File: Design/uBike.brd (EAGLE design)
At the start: 55 x 85 mm, 86 parts, among them J10 455-1750-1-ND, J5 C167321, J6 C111196, J9 CONN_08, Q1 B772, Q2 B772, U1 RA-02_LORA, U10 MAX17048, U2 RP2040, U3 W25Q128JVSIQ, U5 PAM2401, U6 AMS1117-3.3, U8 MCP73831, Y1 12MHz

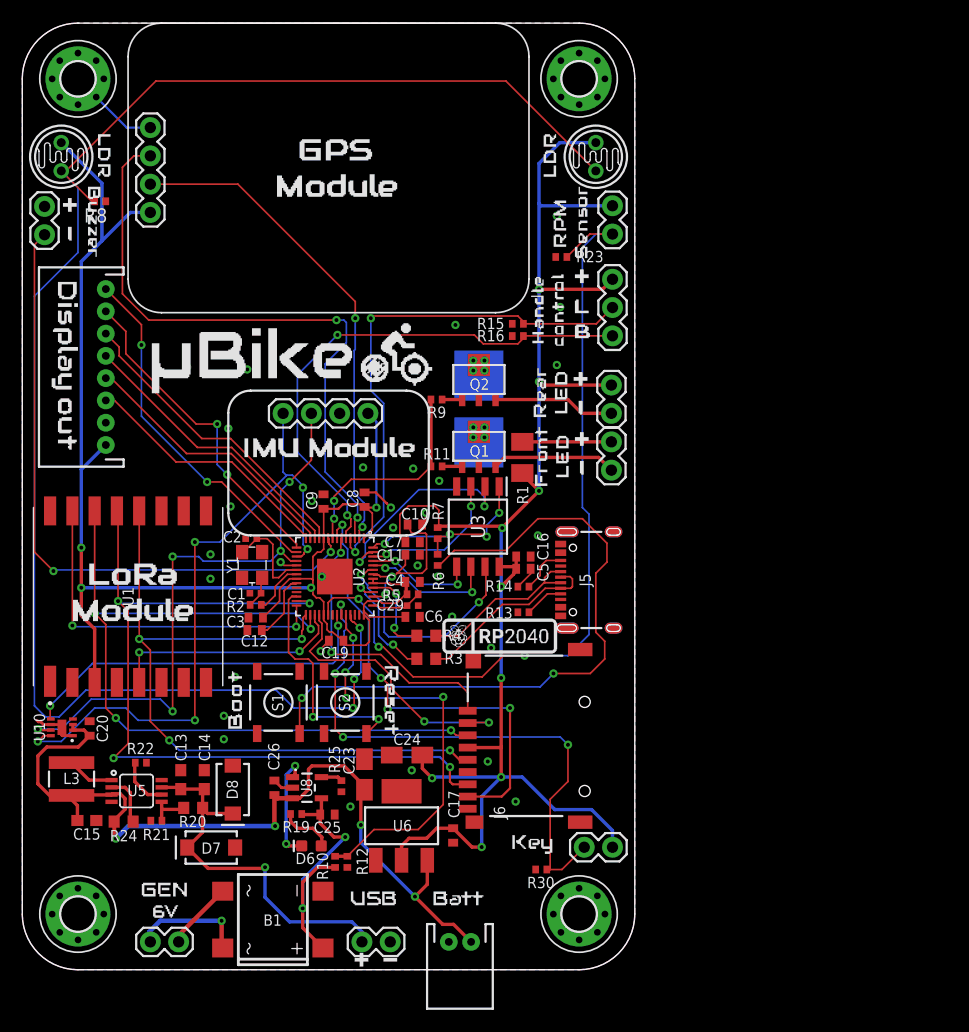
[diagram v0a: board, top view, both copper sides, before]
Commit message: Frozen design for August 23 manufacturing batch
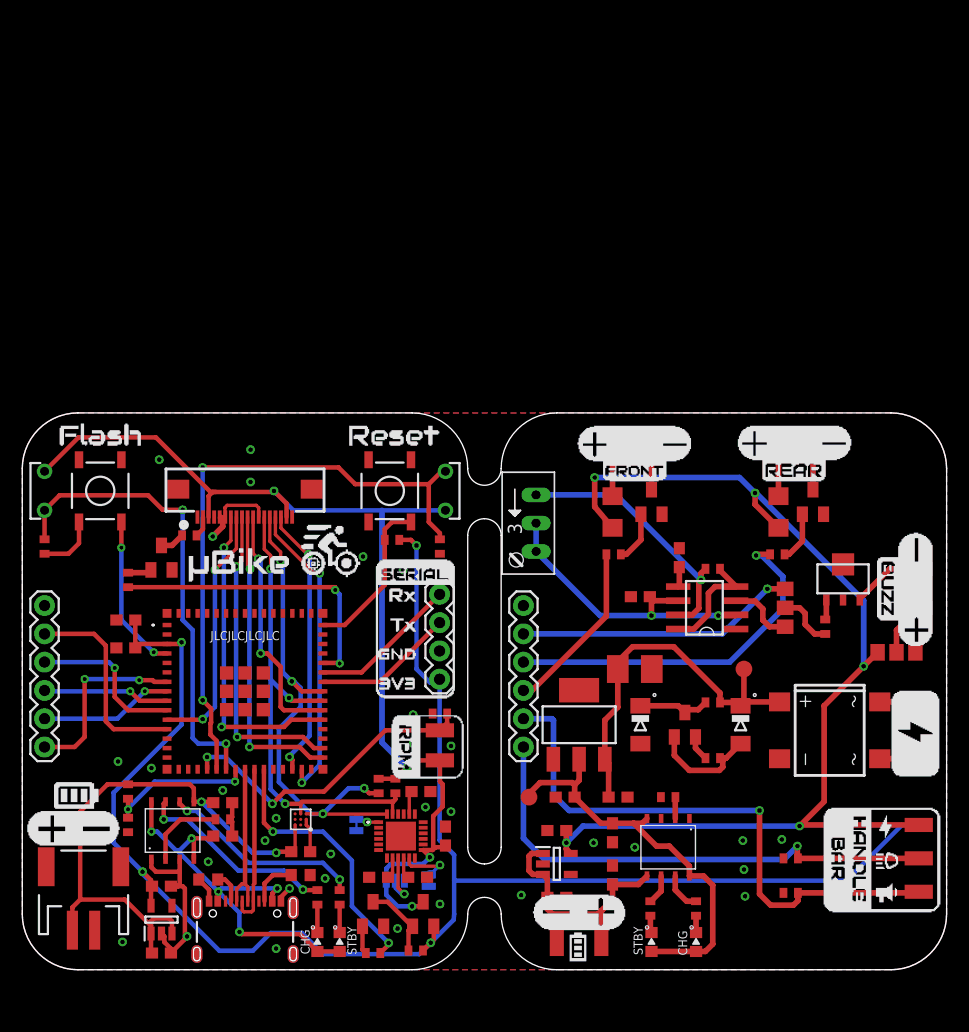
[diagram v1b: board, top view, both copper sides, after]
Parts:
- removed C20: 100nF, rcl:C0402
- removed C23, C24: 10uF, rcl:A/3216-18R
- removed C25, C26: 4.7uF, rcl:C0402
- removed C29: 2.2uF, SparkFun-Capacitors:0402-TIGHT
- removed D6: Yellow, SparkFun-LED:LED-0603
- removed D7, D8: B340A, SparkFun-DiscreteSemi:SMA-DIODE
- removed H1, H2, H3, H4: MOUNT-PAD-ROUND, SpaceDIY_connectors:3,0-PAD
- removed J10: 455-1750-1-ND, SparkFun-Connectors:1X03
- removed J11, J12, J13, J2, J3, J8: (no value), SparkFun-Connectors:1X02
- removed J14: (no value), SparkFun-Connectors:1X04
- removed J6: C111196, SparkFun-Connectors:MICROSD-EXTERNALPIN
- removed J9: CONN_08, SpaceDIY_connectors:JST-8-PTH
- removed L3: 2.2UH3A, SparkFun-Coils:INDUCTOR_4X4MM
- removed Q1, Q2: B772, User-Submitted:SOT89
- removed R30: 10k, rcl:R0402
- removed U$30: (no value), RP2040:RP2040_20
- removed U10: MAX17048, SparkFun-IC-Power:DFN-8
- removed U2: RP2040, RP2040:QFN-56
- removed U3: W25Q128JVSIQ, SamacSys_Parts:SOIC127P790X216-8N
- removed U5: PAM2401, SparkFun-IC-Power:MSOP8
- removed U6: AMS1117-3.3, SparkFun-IC-Power:SOT223
- removed U8: MCP73831, SparkFun-IC-Power:SOT23-5
- removed Y1: 12MHz, crystal-geyer_V1_0:3.2X2.5_KX-7
- added C18: 10uF, rcl:C0603
- added C40: 1uF, rcl:C0603
- added D1, D2: ZMM5V6-M, JLC PCB Basic Parts_loc:MELF-MLL34
- added IC1, IC4: TP4056, TP4056:SOT23-8
- added IC2, IC7: RT9080-33GJ5, SamacSys_Parts:SOT94P280X100-5N
- added IC3: MPU-6050, SpaceDIY_IC:MPU6050
- added IC5: LC709203F/MH, adafruit_sensor:WLCSP9
- added IC6: ESP32-S3-MINI-1U-N8, SpaceDIY_modules:ESP32S3MINI1UN8
- added IC8: TLC555CDR, adafruit:SO08
- added J18: (no value), SparkFun-Connectors:1X04
- added JMP1, JMP2: 0R-JUMPA, jump-0r-smd:A0R-JMP
- added LED1, LED3: Red, SpaceDIY_semiconductors:LED_0603
- added LED2, LED4: Green, SpaceDIY_semiconductors:LED_0603
- added PAD1, PAD10, PAD11, PAD12, PAD13, PAD14, PAD15, PAD2, PAD3, PAD4, PAD5, PAD6, PAD7, PAD8, PAD9: (no value), wirepad:SMD1,27-2,54
- added Q5: B772, User-Submitted:SOT89
- added R17, R28: 1k, SpaceDIY_passive_components:0402
- added R18: 10K, SpaceDIY_passive_components:0402
- added R26: 1.2k, SpaceDIY_passive_components:0402
- added R27: 1K, SpaceDIY_passive_components:0402
- added R29: 1M, SpaceDIY_passive_components:0402
- added R36, R37: 5.1k, rcl:R0603
- added SJ1: (no value), SparkFun:SJ_3_PASTE2&3
- added SJ2, SJ3: (no value), SparkFun:SJ_2S-TRACE
- added T1, T6: MMBT2222A, JLC PCB Basic Parts_loc:SOT23
- added T2: T_P-MOSFET_SI2301CDS-T1-GE3_VISHAY_SOT23-GSD, JLC PCB Basic Parts_loc:SOT23
- added T3, T4, T5: T_N-MOSFET_2N7002_CHANGJ_SOT23-GSD, JLC PCB Basic Parts_loc:SOT23
- added TP1, TP3: TPTP15R, testpad:TP15R
- added U$1: P169H002-CTP, SpaceDIY_connectors:FPC_18_0.5MM_BOTTOM
- C1: value 15pF -> 10uF; device SparkFun-Capacitors:0402-TIGHT -> rcl:C0603
- C10, C17, C4, C7, C8: value 100nF -> 10uF; device rcl:C0402 -> rcl:C0603
- C11: value 0.1uF -> 100nF; device rcl:C0402 -> rcl:C0603
- C12: value 2.2uF -> 2.2nF; device rcl:C0402 -> rcl:C0603
- C13, C15: value 22uF -> 0.1uF
- C14: value 22uF -> 10nF
- C16, C19: value 2.2uF -> 10uF; device rcl:C0402 -> rcl:C0603
- C2: value 15pF -> 100u; device SparkFun-Capacitors:0402-TIGHT -> SpaceDIY_passive_components:B/3528-21R
- C3: value 100nF -> 10u; device rcl:C0402 -> rcl:C0603
- C5: value 100nF -> 100n; device rcl:C0402 -> rcl:C0603
- C6: value 100nF -> 0.1uF; device rcl:C0402 -> rcl:C0603
- C9: value 100nF -> 10nF; device rcl:C0402 -> rcl:C0603
- J1: device SparkFun-Connectors:1X04 -> SpaceDIY_connectors:JST-2-SMD
- J4: device SparkFun-Connectors:1X02 -> SpaceDIY_connectors:1X06
- J5: value C167321 -> (none); device SparkFun-Connectors:USB-C-16P-4LAYER-ISOLATED -> SpaceDIY_connectors:1X06
- J7: value (none) -> USB-C; device SparkFun-Connectors:JST-2-PTH -> SparkFun-Connectors:USB-C-16P-4LAYER-ISOLATED
- PH1, PH2: value VT20N1 -> M9960_11A; device photo-elements:TO46-VT200 -> photo-elements:M9960
- R1: device rcl:M1206 -> rcl:R1206
- R10, R11, R15, R16, R23, R8, R9: device rcl:R0402 -> SpaceDIY_passive_components:0402
- R12: value 1k -> 1; device rcl:R0402 -> rcl:R1206
- R13: value 5.1k -> 10K; device rcl:R0402 -> SpaceDIY_passive_components:0402
- R14: value 5.1k -> 100; device rcl:R0402 -> SpaceDIY_passive_components:0402
- R19: value 1k -> (none); device rcl:R0402 -> pot:RJ9W
- R2: value 1k -> 10k; device rcl:R0402 -> SpaceDIY_passive_components:0402
- R20: value 750K -> 10K; device rcl:R0603 -> SpaceDIY_passive_components:0402
- R21: value 100k -> 10R; device rcl:R0402 -> SpaceDIY_passive_components:0402
- R22: value 100k -> 1k; device rcl:R0402 -> SpaceDIY_passive_components:0402
- R24: value 750K -> 10k; device rcl:R0603 -> SpaceDIY_passive_components:0402
- R25: value 2k -> 1M; device rcl:R0402 -> SpaceDIY_passive_components:0402
- R3: value 27 -> 1k; device rcl:R0603 -> SpaceDIY_passive_components:0402
- R4: value 27 -> 100; device rcl:R0603 -> SpaceDIY_passive_components:0402
- R5: value 200 -> 10k; device rcl:R0402 -> SpaceDIY_passive_components:0402
- R6: value 1k -> 1.2k; device rcl:R0402 -> SpaceDIY_passive_components:0402
- R7: value 10k -> 1K; device rcl:R0402 -> SpaceDIY_passive_components:0402
- S1: value MOMENTARY-SWITCH-SPST-SMD-5.2MM-TALL -> Flash; device SparkFun-Switches:TACTILE_SWITCH_SMD_5.2MM -> SpaceDIY_electromechanical:TACTILE_SWITCH_SMD_5.2MM
- S2: value MOMENTARY-SWITCH-SPST-SMD-5.2MM-TALL -> Reset; device SparkFun-Switches:TACTILE_SWITCH_SMD_5.2MM -> SpaceDIY_electromechanical:TACTILE_SWITCH_SMD_5.2MM
- U1: value RA-02_LORA -> AMS1117-5VSMD; device SpaceDIY_modules:MODULE_RA-02_LORA -> SpaceDIY_IC:SOT223
- moved J1 60.8 mm to (5.50, 7.50), turned to 180 degrees
- moved PH1 57.9 mm to (2.00, 43.0)
- moved R16 55.7 mm to (69.0, 6.90)
- moved R15 53.9 mm to (69.0, 10.0)
- moved B1 52.8 mm to (72.5, 21.5), turned to 270 degrees
- moved R12 49.9 mm to (67.9, 41.1), turned to 90 degrees
- moved PH2 45.7 mm to (38.0, 43.0), turned to 90 degrees
- moved R23 42.4 mm to (37.5, 23.0)
- moved U1 42.1 mm to (50.0, 22.0), turned to 0 degrees
- moved R7 40.9 mm to (60.5, 5.50)
- moved C1 40.8 mm to (53.0, 8.50), turned to 90 degrees
- moved C8 39.7 mm to (48.0, 6.50), turned to 0 degrees
- moved R24 37.6 mm to (37.5, 38.0), turned to 90 degrees
- moved C2 36.4 mm to (55.0, 27.0), turned to 180 degrees
- moved C3 36.3 mm to (53.5, 15.5), turned to 0 degrees
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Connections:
- removed net !RESET!: S2.3, U2.26
- removed net 1.1V: C10.1, C11.1, C12.1, U2.23, U2.45, U2.50
- removed net ADC0: R10.1, R12.1, U2.38
- removed net ADC1: PH1.2, PH2.2, R8.2, U2.39
- removed net ADC2: U2.40
- removed net ADC3: U2.41
- removed net AVDD: C29.1, R5.1, U2.43
- removed net BATT_ALERT: U10.5, U2.36
- removed net BOOT: R6.2, S1.3
- removed net DAT1: J6.8, U2.7
- removed net DAT2: J6.1, U2.6
- removed net EN_5: R24.1, U5.2
- removed net GPIO2: J10.2, R15.2, U2.4
- removed net GPIO20: U1.5, U2.31
- removed net GPIO21: J6.2, U2.32
- removed net GPIO22: J11.2, R23.2, U2.34
- removed net GPIO23: U2.35
- removed net GPIO25: J13.2, R30.2, U2.37
- removed net GPIO3: J10.3, R16.2, U2.5
- removed net GPIO6: R11.2, R9.2, U2.8
- removed net GPIO7: J12.1, U2.9
- removed net LCD_BL: J9.8, U2.16
- removed net LCD_RST: J9.7, U2.15
- removed net N$24: R20.1, R21.2, U5.5
- removed net N$25: L3.P$2, U5.1
- removed net N$26: R22.2, U5.6
- removed net QSPI-0: U2.53, U3.5
- removed net QSPI-1: U2.55, U3.2
- removed net QSPI-2: U2.54, U3.3
- removed net QSPI-3: U2.51, U3.7
- removed net QSPI-CLK: U2.52, U3.6
- removed net QSPI-CS: R6.1, R7.1, U2.56, U3.1
- removed net RX_GPS: J1.2, U2.2
- removed net SPI_0_CS: U1.15, U2.28
- removed net SPI_0_MISO: J6.7, U1.13, U2.27
- removed net SPI_0_MOSI: J6.3, U1.14, U2.30
- removed net SPI_0_SCK: J6.5, U1.12, U2.29
- removed net SPI_1_CS: J9.5, U2.12
- removed net SPI_1_MISO: J9.6, U2.11
- removed net SPI_1_MOSI: J9.3, U2.14
- removed net SPI_1_SCK: J9.4, U2.13
- removed net SWDCK: U2.24
- removed net SWDIO: U2.25
- removed net TX_GPS: J1.3, U2.3
- removed net USB_F_N1: R3.2, U2.46
- removed net USB_F_P1: R4.2, U2.47
- removed net USB_N: J5.A7, J5.B7, R3.1
- removed net USB_P: J5.A6, J5.B6, R4.1
- removed net V_BATT: C15.1, C20.1, C23.+, C26.1, J7.1, L3.P$1, R24.2, U10.2, U10.3, U5.3, U6.3, U8.3
- removed net V_IN: B1.+, C25.1, R10.2, R19.2, U8.4
- new net BAT_VOLT: IC6.22, R25.1, R29.2
- new net BUZZER: JMP2.2, R14.2
- new net BUZZ_PB: IC6.8, J4.2, J5.2, PAD15.1, R16.2
- new net CC3: J7.B5, R36.2
- new net CC4: J7.A5, R37.2
- new net D+: IC6.24, J7.A6, J7.B6
- new net D-: IC6.23, J7.A7, J7.B7
- new net IO0: IC6.4, S1.3
- new net LDR_LH: IC6.21, PH1.2, R8.2
- new net LDR_RH: IC6.20, PH2.2, R24.2
- new net LEDK: R21.1, U$1.2
- new net LED_FRONT: IC6.9, J4.3, J5.3, R11.2
- new net LED_PB: IC6.7, J4.1, J5.1, PAD14.1, R15.2
- new net LED_REAR: IC6.10, J4.4, J5.4, R9.2
- new net N$15: IC1.7, R7.2
- new net N$17: PAD12.1, Q5.3
- new net N$18: R3.2, T1.1
- new net N$19: JMP1.2, PAD11.1
- new net N$20: PAD1.1, R12.2
- new net N$33: R21.2, T6.3
- new net N$34: IC8.7, R17.2, R19.E
- new net N$35: C11.1, IC8.2, IC8.6, R19.A, R19.S
- new net N$36: IC8.3, JMP2.1
- new net N$37: C9.1, IC8.5
- new net N$38: IC3.11, SJ3.2
- new net N$39: IC3.1, SJ2.2
- new net N$40: C13.1, IC3.10
- new net N$41: C12.1, IC3.20
- new net N$43: C14.1, IC3.8
- new net N$44: IC3.9, SJ1.2
- new net N$46: R22.2, T6.1
- new net N$47: IC4.6, R28.2
- new net N$48: LED3.C, R27.1
- new net N$49: LED4.C, R28.1
- new net N$50: IC4.2, R26.2
- new net N$51: IC4.7, R27.2
- new net RPM: IC6.19, PAD10.1, R23.2
- new net RST: IC6.45, R13.1, S2.3
- new net RX: IC6.6
- new net RXD0: IC6.40, J18.4
- new net SENS: IC6.25, R3.1
- new net TFT_BL: IC6.41, R22.1
- new net TFT_CS: IC6.11, U$1.8
- new net TFT_DC: IC6.35, U$1.7
- new net TFT_MISO: IC6.33
- new net TFT_MOSI: IC6.31, U$1.10
- new net TFT_RST: IC6.36, U$1.11
- new net TFT_SCK: IC6.32, U$1.9
- new net TP_INT: IC6.28, U$1.16
- new net TP_RST: IC6.29, U$1.15
- new net TX: IC6.5
- new net TXD0: IC6.39, J18.3
- new net UC_BUZZER: IC6.12, J4.5, J5.5, JMP2.3
- new net VBAT: C16.1, C18.1, C40.1, IC4.5, IC5.A3, IC7.1, IC7.3, J1.1, R25.2
- new net VBAT_1: C1.1, C8.1, IC1.5, IC2.1, IC2.3, PAD5.1
- new net VBUS: C17.1, IC4.4, IC4.8, J7.VBUS1, J7.VBUS2, LED3.A, LED4.A
- new net VSENS: C15.1, IC3.13, PAD9.1, PH1.1, PH2.1, R18.1, R20.1, SJ1.1, T2.3, U$1.17, U$1.3
- new net V_BUZZ: IC8.4, IC8.8, R17.1
- new net V_DYN_UR: B1.+, C2.+, C3.1, D2.C, R4.1, TP1.TP, U1.3
- new net V_REG: C4.1, C5.1, IC1.4, IC1.8, LED1.A, LED2.A, TP3.TP, U1.2
- net 3.3V: now also C10.1, IC2.5, IC6.3, IC7.5, J18.1, JMP1.3, PAD13.1, R12.1, R13.2, R2.1, T2.2; no longer C16.1, C17.1, C24.+, C3.1, C4.1, C5.1, C8.1, C9.1, J1.1, J10.1, J11.1, J13.1, J14.1, J3.1, J6.4, J9.1, PH1.1, PH2.1, R5.2, R7.2, U1.3, U2.1, U2.10, U2.22, U2.33, U2.42, U2.44, U2.48, U2.49, U3.8, U6.2
- net 5V: now also JMP1.1; no longer C13.1, C14.1, D7.C, D8.C, J4.1, R20.2, U5.7
- net GND: now also C1.2, C18.2, C2.-, C40.2, D1.A, IC1.1, IC1.3, IC2.2, IC3.18, IC4.1, IC4.3, IC5.A1, IC5.B1, IC6.1, IC6.2, IC6.42, IC6.43, IC6.46, IC6.47, IC6.48, IC6.49, IC6.50, IC6.51, IC6.52, IC6.53, IC6.54, IC6.55, IC6.56, IC6.57, IC6.58, IC6.59, IC6.60, IC6.61, IC6.62, IC6.63, IC6.64, IC6.65, IC6.66, IC6.67, IC6.68, IC6.69, IC6.70, IC6.71, IC6.72, IC6.73, IC7.2, IC8.1, J1.2, J18.2, J4.6, J5.6, J7.GND, J7.GND2, PAD6.1, Q5.2, R24.1, R26.1, R29.1, R36.1, R37.1, R5.2, R6.1, SJ1.3, SJ2.1, SJ3.1, T1.2, T3.2, T4.2, T5.2, T6.2, U$1.1, U$1.12, U$1.18, U$1.5, U$1.6; no longer C1.1, C2.1, C20.2, C23.-, C24.-, C25.2, C26.2, C29.2, D7.A, D8.A, H1.B3,0, H1.P$2, H1.P$3, H1.P$4, H1.P$5, H1.P$6, H1.P$7, H1.P$8, H1.P$9, H2.B3,0, H2.P$2, H2.P$3, H2.P$4, H2.P$5, H2.P$6, H2.P$7, H2.P$8, H2.P$9, H3.B3,0, H3.P$2, H3.P$3, H3.P$4, H3.P$5, H3.P$6, H3.P$7, H3.P$8, H3.P$9, H4.B3,0, H4.P$2, H4.P$3, H4.P$4, H4.P$5, H4.P$6, H4.P$7, H4.P$8, H4.P$9, J1.4, J12.2, J14.2, J4.2, J5.GND, J5.GND2, J6.10, J6.11, J6.12, J6.13, J6.6, J6.9, J7.2, J9.2, Q1.2, Q2.2, R12.2, R13.2, R14.2, R21.1, R22.1, R25.1, R30.1, U1.16, U1.2, U1.9, U10.1, U10.4, U10.6, U10.9, U2.19, U2.EPAD, U3.4, U5.4, U5.8, U6.1, U8.2
- net N$1: now also PAD3.1; no longer J2.1
- net N$10: now also PAD8.1; no longer J8.2
- net N$11: now also LED1.C, R7.1; no longer D6.A, R19.1
- net N$12: now also LED2.C, R10.1; no longer J5.B5, R14.1
- net N$13: now also IC1.2, R6.2; no longer D6.C, U8.1
- net N$14: now also PAD7.1; no longer J8.1
- net N$16: now also Q5.1, R14.1; no longer R25.2, U8.5
- net N$2: now also T4.1; no longer Q2.1
- net N$3: now also IC1.6, R10.2; no longer R2.2, U2.21
- net N$4: now also PAD4.1, T3.3; no longer J2.2, Q1.3
- net N$5: now also T3.1; no longer Q1.1
- net N$6: now also PAD2.1, T4.3; no longer J3.2, Q2.3
- net N$7: now also D2.A, R5.1, T5.1; no longer C2.2, U2.20, Y1.3
- net N$8: now also D1.C, R4.2, T5.3; no longer C1.2, R2.1, Y1.1
- net N$9: now also R2.2, T1.3, T2.1; no longer J5.A5, R13.1
- net SCL: now also IC3.23, IC5.C2, IC6.37, R18.2, U$1.13; no longer J14.3, U10.7, U2.18
- net SDA: now also IC3.24, IC5.C1, IC6.38, R20.2, U$1.14; no longer J14.4, U10.8, U2.17
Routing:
- net ADC1: track 148.9 -> 0.00 mm, vias 3 -> 0
- net VSENS: track 0.00 -> 97.9 mm, vias 0 -> 4
- net V_BATT: track 78.3 -> 0.00 mm, vias 4 -> 0
- net SPI_0_MISO: track 75.3 -> 0.00 mm, vias 4 -> 0
- net GPIO22: track 73.8 -> 0.00 mm, vias 3 -> 0
- net SPI_0_MOSI: track 72.9 -> 0.00 mm, vias 4 -> 0
- net SPI_0_SCK: track 66.2 -> 0.00 mm, vias 4 -> 0
- net BUZZ_PB: track 0.00 -> 63.7 mm, vias 0 -> 2
- net LED_PB: track 0.00 -> 62.7 mm, vias 0 -> 3
- net BOOT: track 60.9 -> 0.00 mm, vias 2 -> 0
- net GPIO7: track 58.2 -> 0.00 mm, vias 2 -> 0
- net TX_GPS: track 56.9 -> 0.00 mm, vias 2 -> 0
- net LDR_RH: track 0.00 -> 55.9 mm, vias 0 -> 2
- net VBAT: track 0.00 -> 51.3 mm, vias 0 -> 2
- net GPIO25: track 50.6 -> 0.00 mm, vias 4 -> 0
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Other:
- board size 55 x 85 mm -> 83 x 50 mm
- board text added: "CHG"
- board text added: "JLCJLCJLCJLC"
- board text added: "STBY"
